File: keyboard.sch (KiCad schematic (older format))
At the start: 29 parts, among them J1 USB_MINI-B, J2 Conn_01x02, P1 ISP, P3 GPIO_CLUSTER2, U1 ATMEGA32U4, U2 SPX3819M5-L-3-3, U4 MCP73831, X1 CRYSTAL

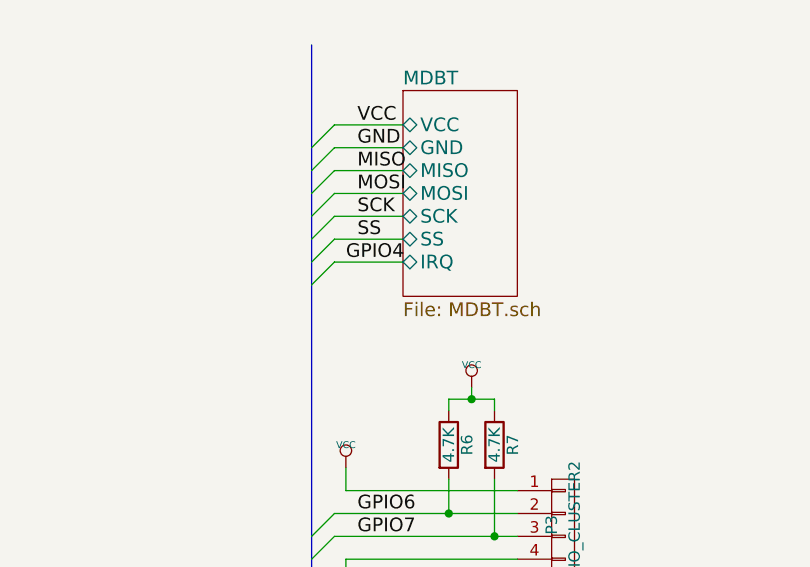
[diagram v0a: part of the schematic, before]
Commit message: 2017年10月29日
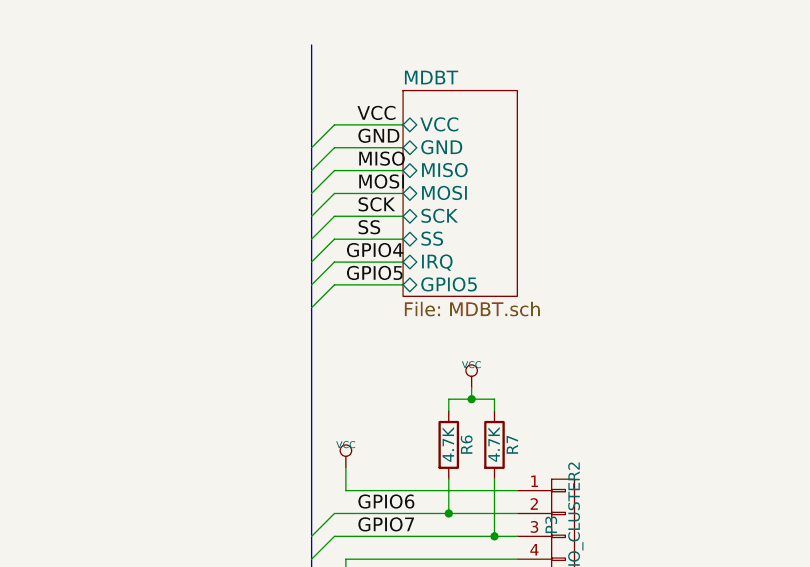
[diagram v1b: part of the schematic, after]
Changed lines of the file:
@@
 F7 "SS" B L 8550 1350 60
 F8 "IRQ" B L 8550 1450 60
+F9 "GPIO5" B L 8550 1550 60
 $EndSheet
 Entry Wire Line
@@
 Connection ~ 2650 2500
 Connection ~ 3000 1200
+Entry Wire Line
+	8150 1650 8250 1550
+Wire Wire Line
+	8250 1550 8550 1550
+Text Label 8300 1550 0    60   ~ 0
+GPIO5
 $EndSCHEMATC
